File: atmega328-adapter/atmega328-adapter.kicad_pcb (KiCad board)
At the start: 2 copper layers, 21.9 x 36.6 mm, 4 parts, among them J1 Conn_01x14, J2 Conn_01x14, U1 ATmega168A-A

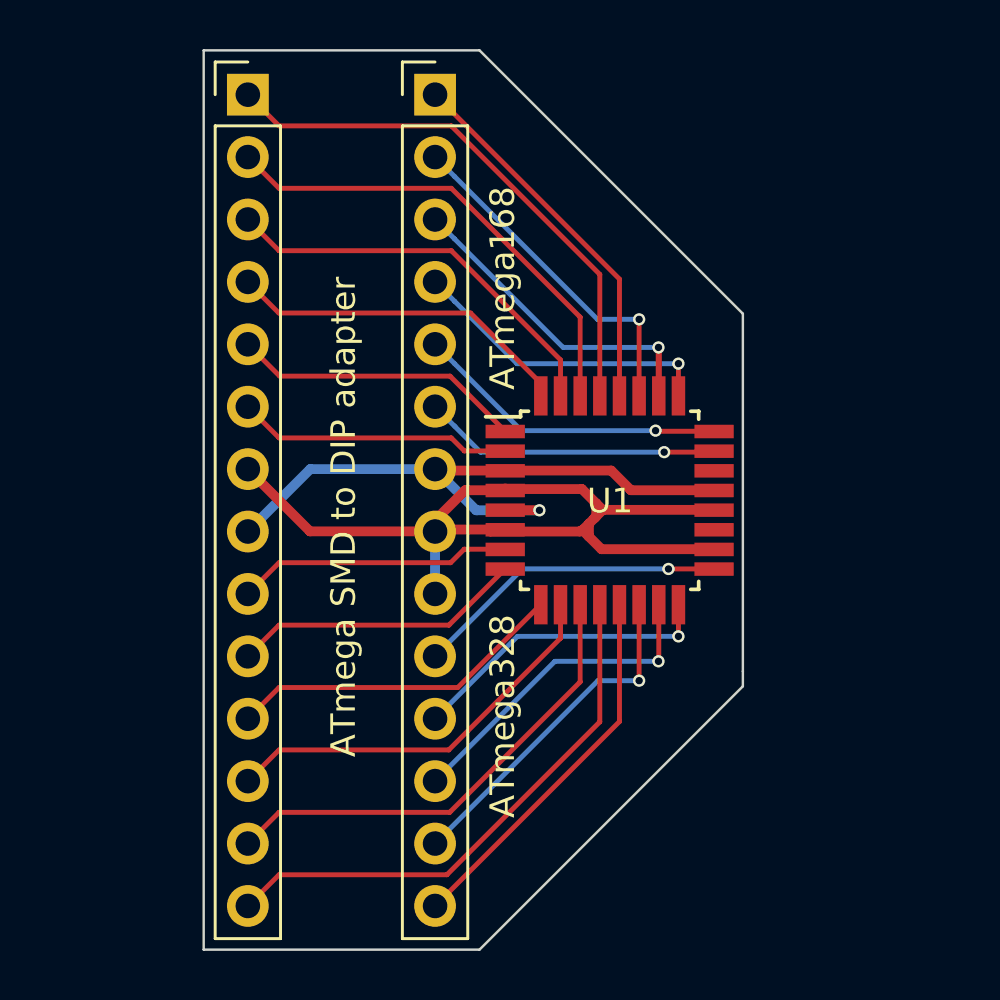
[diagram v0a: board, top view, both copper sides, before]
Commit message: kikit tabs
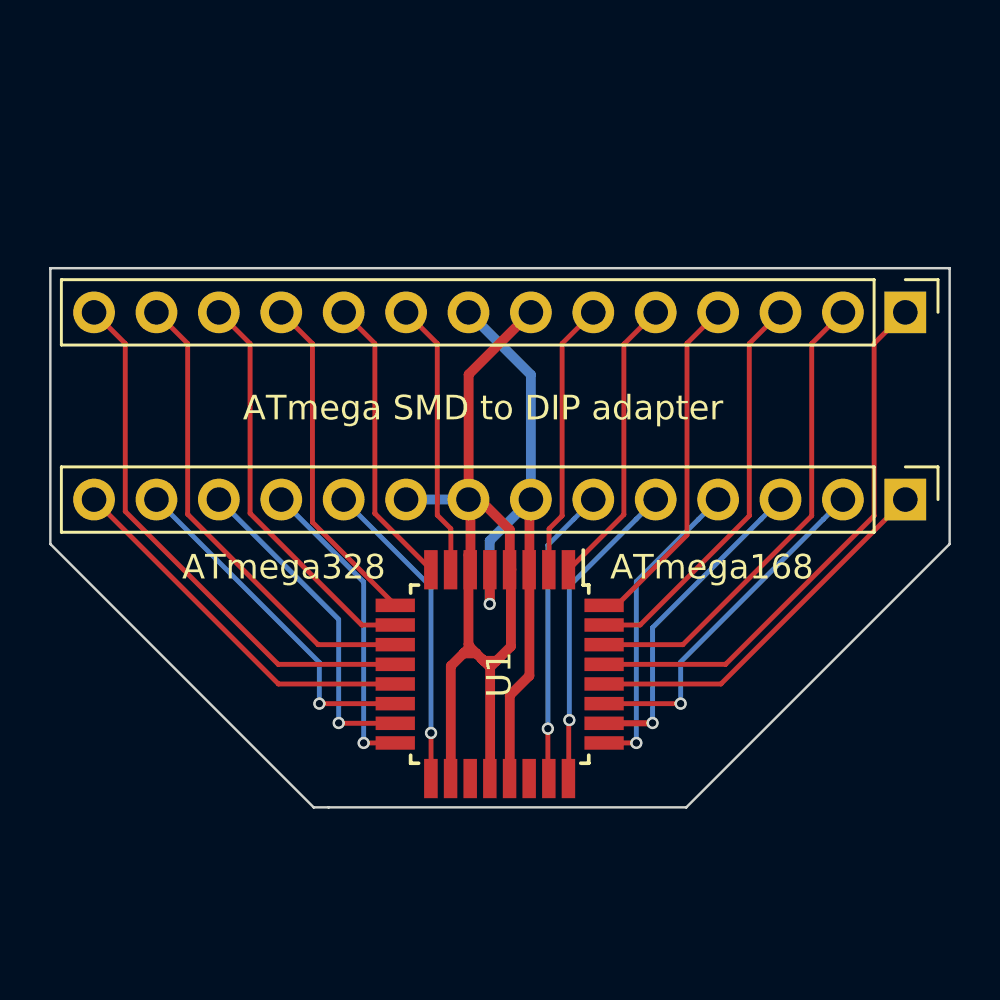
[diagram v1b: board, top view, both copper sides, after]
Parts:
- added REF**: Tab, kikit:Tab, F.Cu at (113.1, 57.3)
- added REF**: Tab, kikit:Tab, F.Cu at (125.5, 79.7)
- added REF**: Tab, kikit:Tab, F.Cu at (143.7, 63.1)
- added REF**: Tab, kikit:Tab, F.Cu at (137.3, 57.2)
- added REF**: Tab, kikit:Tab, F.Cu at (106.6, 63.1)
- moved J1 28.2 mm to (141.7, 59.3), turned to -90 degrees
- moved J2 25.3 mm to (141.7, 66.9), turned to -90 degrees
- moved G*** 8.37 mm to (125.2, 74.0), turned to 180 degrees
- moved U1 8.37 mm to (125.2, 74.0), turned to -90 degrees
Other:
- board size 21.9 x 36.6 mm -> 36.6 x 21.9 mm
